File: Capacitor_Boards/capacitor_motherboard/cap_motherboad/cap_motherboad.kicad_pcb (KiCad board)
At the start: 2 copper layers, 180.5 x 92 mm, 14 parts, among them J1 Conn_01x02_Female, J10 Conn_01x02_Female, J11 Conn_01x02_Female, J12 Conn_01x02_Female, J2 Conn_01x02_Female, J3 Conn_01x02_Female, J4 Conn_01x02_Female, J5 Conn_01x02_Female, J6 Conn_01x02_Female, J7 Conn_01x02_Female, J8 Conn_01x02_Female, J9 Conn_01x02_Female

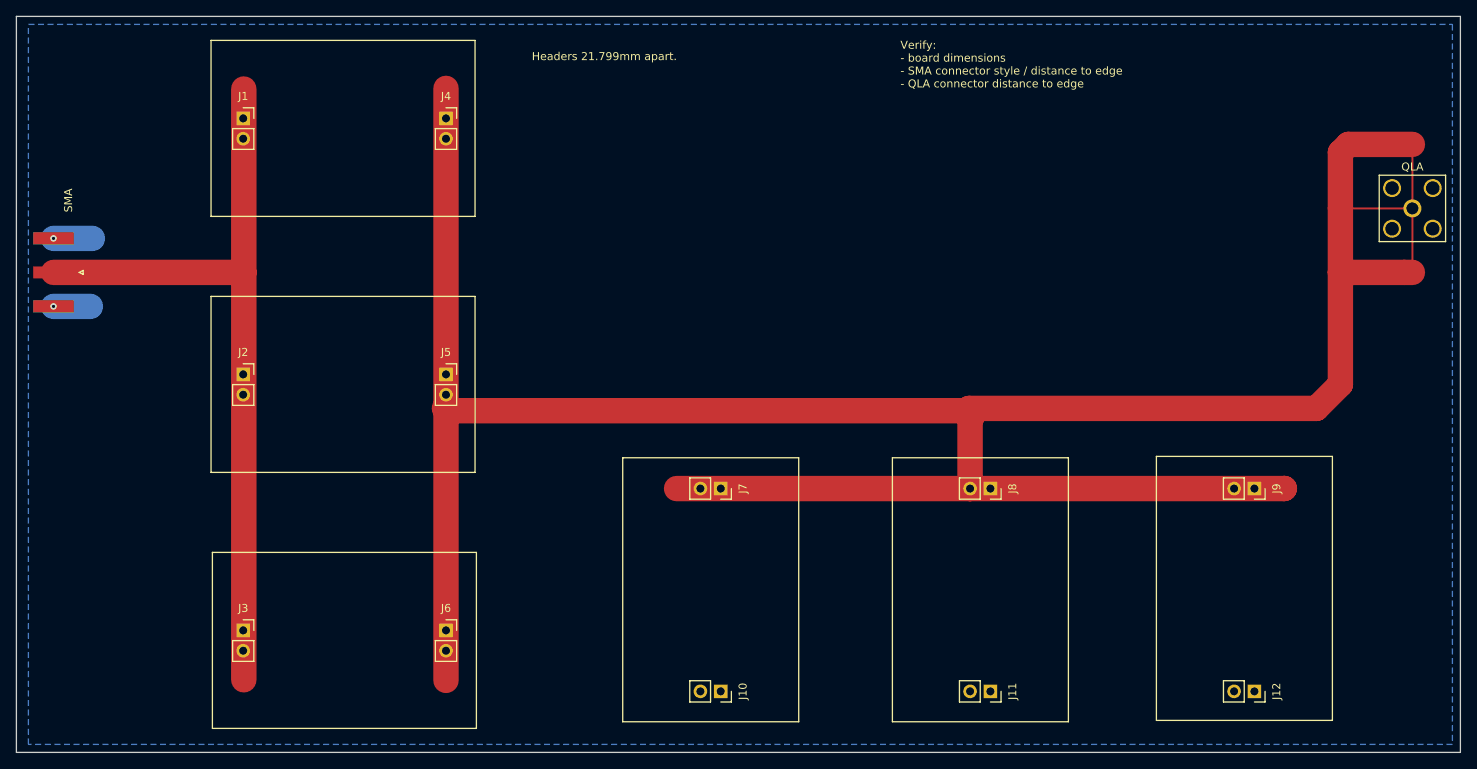
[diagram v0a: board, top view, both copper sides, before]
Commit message: Finalized boards
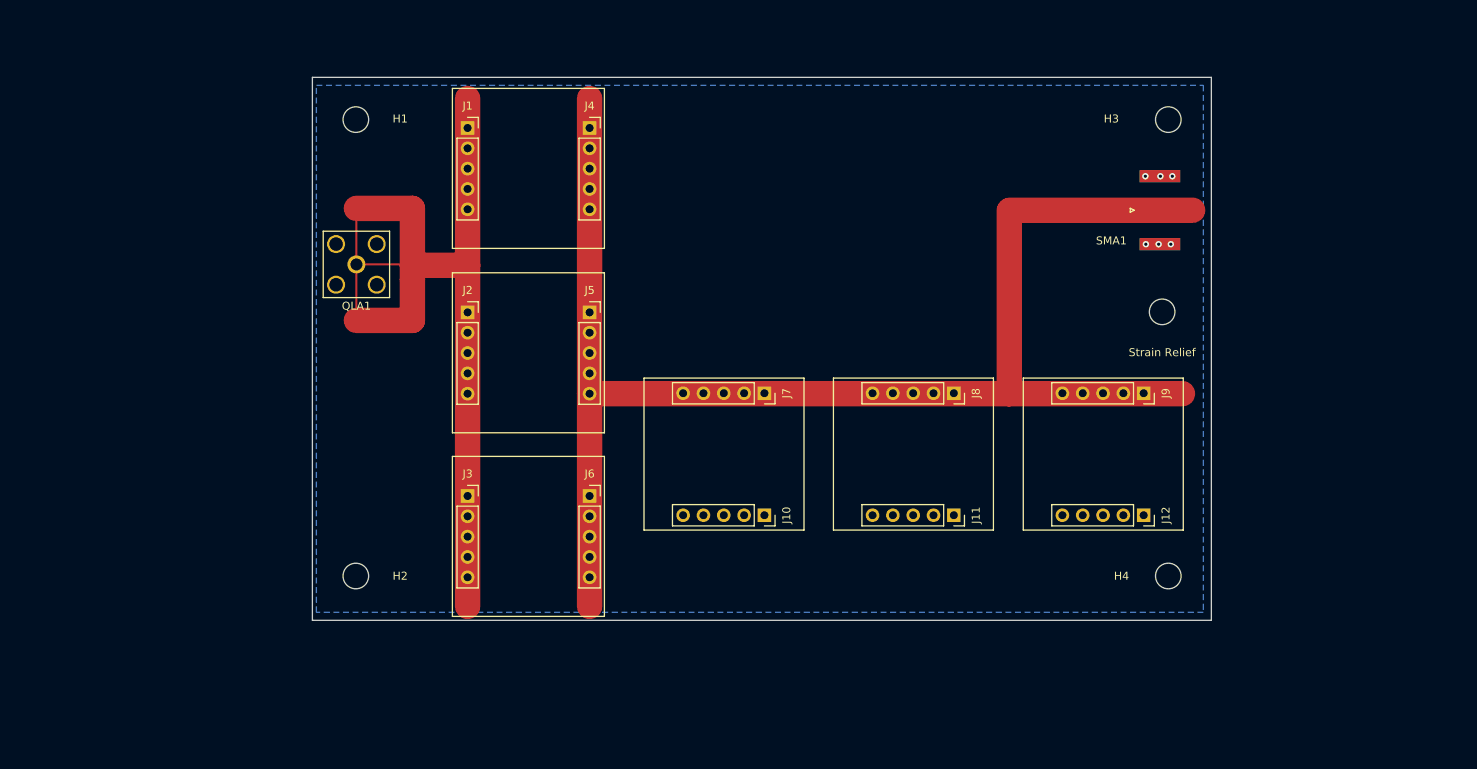
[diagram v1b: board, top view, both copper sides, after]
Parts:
- added H1: MountingHole, MountingHole:MountingHole_3.2mm_M3, F.Cu at (71.9, 50.9)
- added H2: MountingHole, MountingHole:MountingHole_3.2mm_M3, F.Cu at (71.9, 108.0)
- added H3: MountingHole, MountingHole:MountingHole_3.2mm_M3, F.Cu at (173.5, 50.9)
- added H4: MountingHole, MountingHole:MountingHole_3.2mm_M3, F.Cu at (173.5, 108.0)
- added Strain Relief: MountingHole, MountingHole:MountingHole_3.2mm_M3, F.Cu at (172.7, 74.9)
- J1, J10, J11, J12, J2, J3, J4, J5, J6, J7, J8, J9: value Conn_01x02_Female -> Conn_01x05; footprint Connector_PinSocket_2.54mm:PinSocket_1x02_P2.54mm_Vertical -> Connector_PinSocket_2.54mm:PinSocket_1x05_P2.54mm_Vertical
- moved SMA1 138.5 mm to (172.4, 62.2), turned to 0 degrees
- moved QLA1 132.2 mm to (72.0, 69.0), turned to 90 degrees
- moved J3 32.7 mm to (85.9, 98.0)
- moved J2 29.1 mm to (85.9, 75.0)
- moved J1 28.1 mm to (85.9, 52.0)
- moved J12 26.0 mm to (170.4, 100.4)
- moved J6 24.6 mm to (101.2, 98.0)
- moved J10 22.7 mm to (123.0, 100.4)
- moved J11 22.5 mm to (146.7, 100.4)
- moved J5 19.6 mm to (101.2, 75.0)
- moved J9 18.3 mm to (170.4, 85.1)
- moved J4 18.0 mm to (101.2, 52.0)
- moved J7 13.1 mm to (123.0, 85.1)
- moved J8 12.8 mm to (146.7, 85.1)
- renumbered QLA to QLA1, SMA to SMA1
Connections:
- QLA1 pad 1: Net-(J4-Pad1) -> Net-(J1-Pad1)
- SMA1 pad 1: Net-(J1-Pad1) -> Net-(J4-Pad1)
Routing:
- net Net-(J4-Pad1): track 344.6 -> 183.4 mm
- net Net-(J1-Pad1): track 97.6 -> 118.4 mm
- net GND: track 9.47 -> 0.00 mm, vias 2 -> 6
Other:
- board size 180.5 x 92 mm -> 112.4 x 67.9 mm
- board text removed: "Headers 21.799mm apart."
- board text removed: "Verify: - board dimensions - SMA connector style / distance to edge - QLA connector distance to edge"
